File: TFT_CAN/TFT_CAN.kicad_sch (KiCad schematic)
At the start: 9 parts, among them J1 Conn_01x20, J2 Conn_01x20, SW1 Conn_01x02, SW2 Conn_01x02

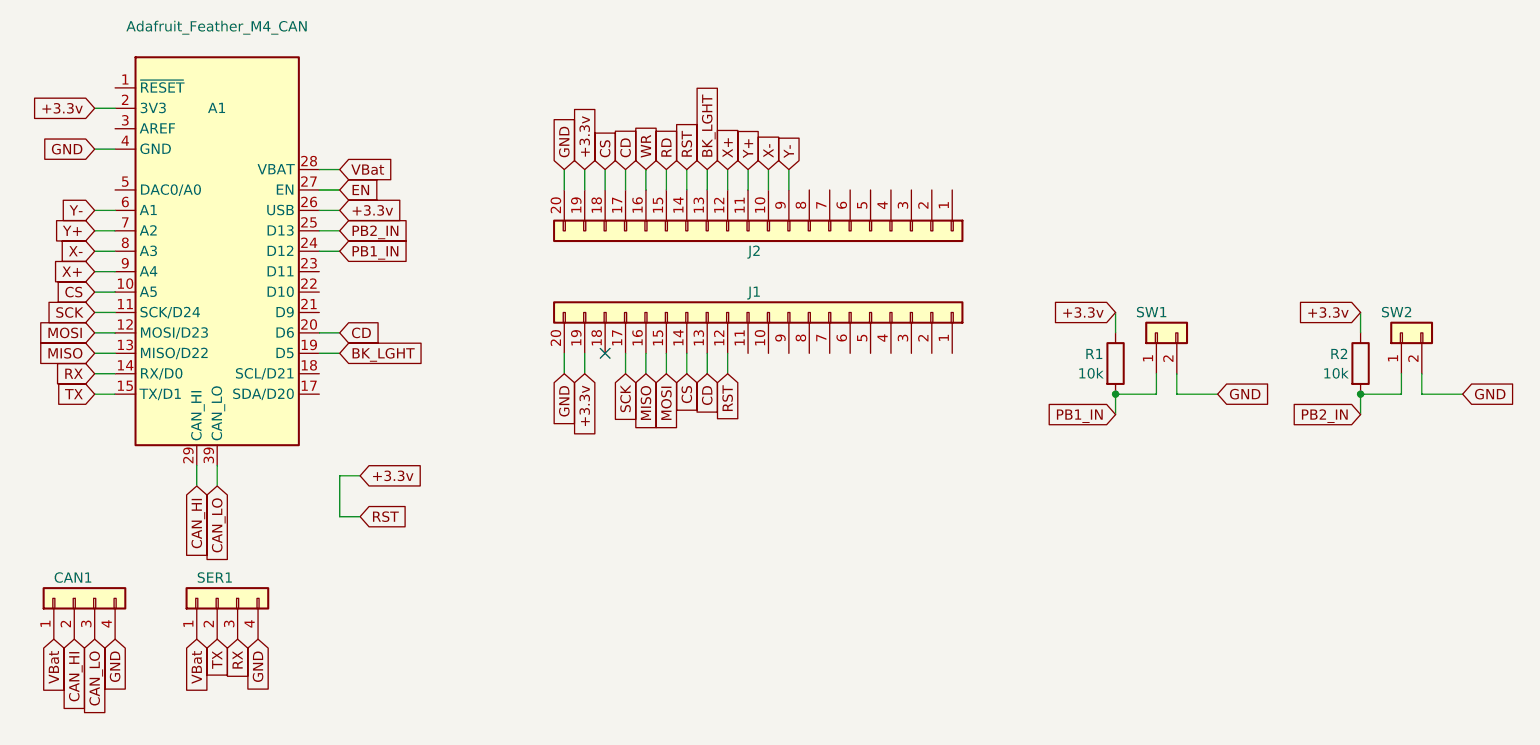
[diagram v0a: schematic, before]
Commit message: finished layout
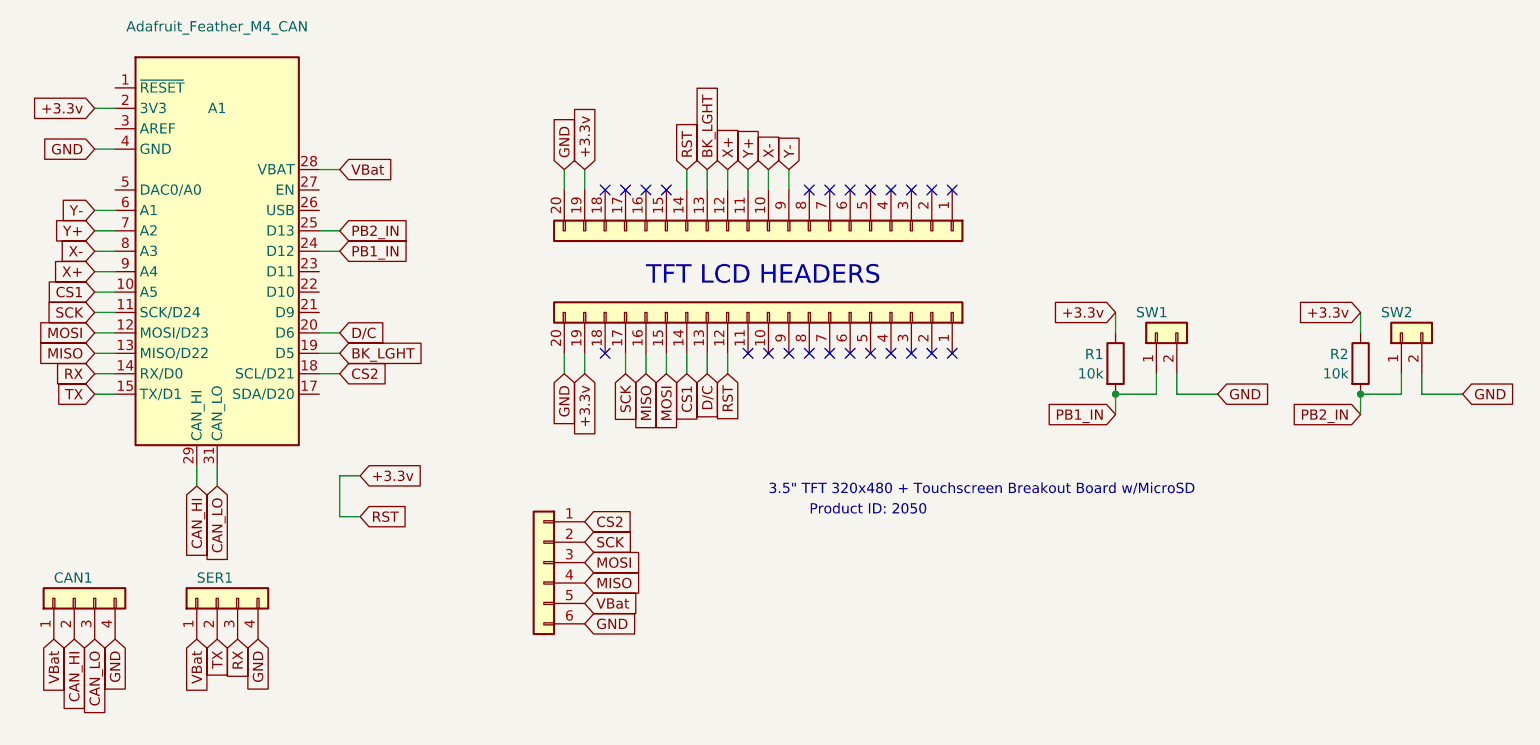
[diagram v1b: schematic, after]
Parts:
- added J3: Conn_01x06, Connector_PinHeader_2.54mm:PinHeader_1x06_P2.54mm_Vertical, symbol Connector_Generic:Conn_01x06
- A1: footprint Module:Adafruit_Feather -> Module:Adafruit_Feather_M4_CAN
- CAN1: footprint Connector_PinHeader_2.54mm:PinHeader_1x04_P2.54mm_Vertical -> Connector_PinHeader_2.54mm:my_4_tab_edge
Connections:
- net +3.3v: no longer A1.26 (USB)
- net CAN_LO: now also A1.31 (CAN_LO); no longer A1.39 (CAN_LO)
- net GND: now also J3.6 (Pin_6)
- net MISO: now also J3.4 (Pin_4)
- net MOSI: now also J3.3 (Pin_3)
- net SCK: now also J3.2 (Pin_2)
- net VBat: now also J3.5 (Pin_5)
- net CS2: now reaches A1.18 (SCL/D21)
- net CS2: now also J3.1 (Pin_1)
- net CD renamed D/C
- net D/C: no longer J2.17 (Pin_17)
- net CS renamed CS1
- net CS1: no longer J2.18 (Pin_18)
- net EN: no longer names the net of A1.27 (EN)
- net RD: no longer names the net of J2.15 (Pin_15)
- net WR: no longer names the net of J2.16 (Pin_16)
- no-connect marks 1 -> 24
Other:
- note added: "3.5" TFT 320x480 + Touchscreen Breakout Board w/MicroSD"
- note added: "Product ID: 2050"
- note added: "TFT LCD HEADERS"
